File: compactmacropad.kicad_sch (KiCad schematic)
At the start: 31 parts, among them SW1 RotaryEncoder_Switch, SW3 RotaryEncoder_Switch, U1 MCU_Seeed_XIAO_RP2040, U2 SN74LV1T34DBV

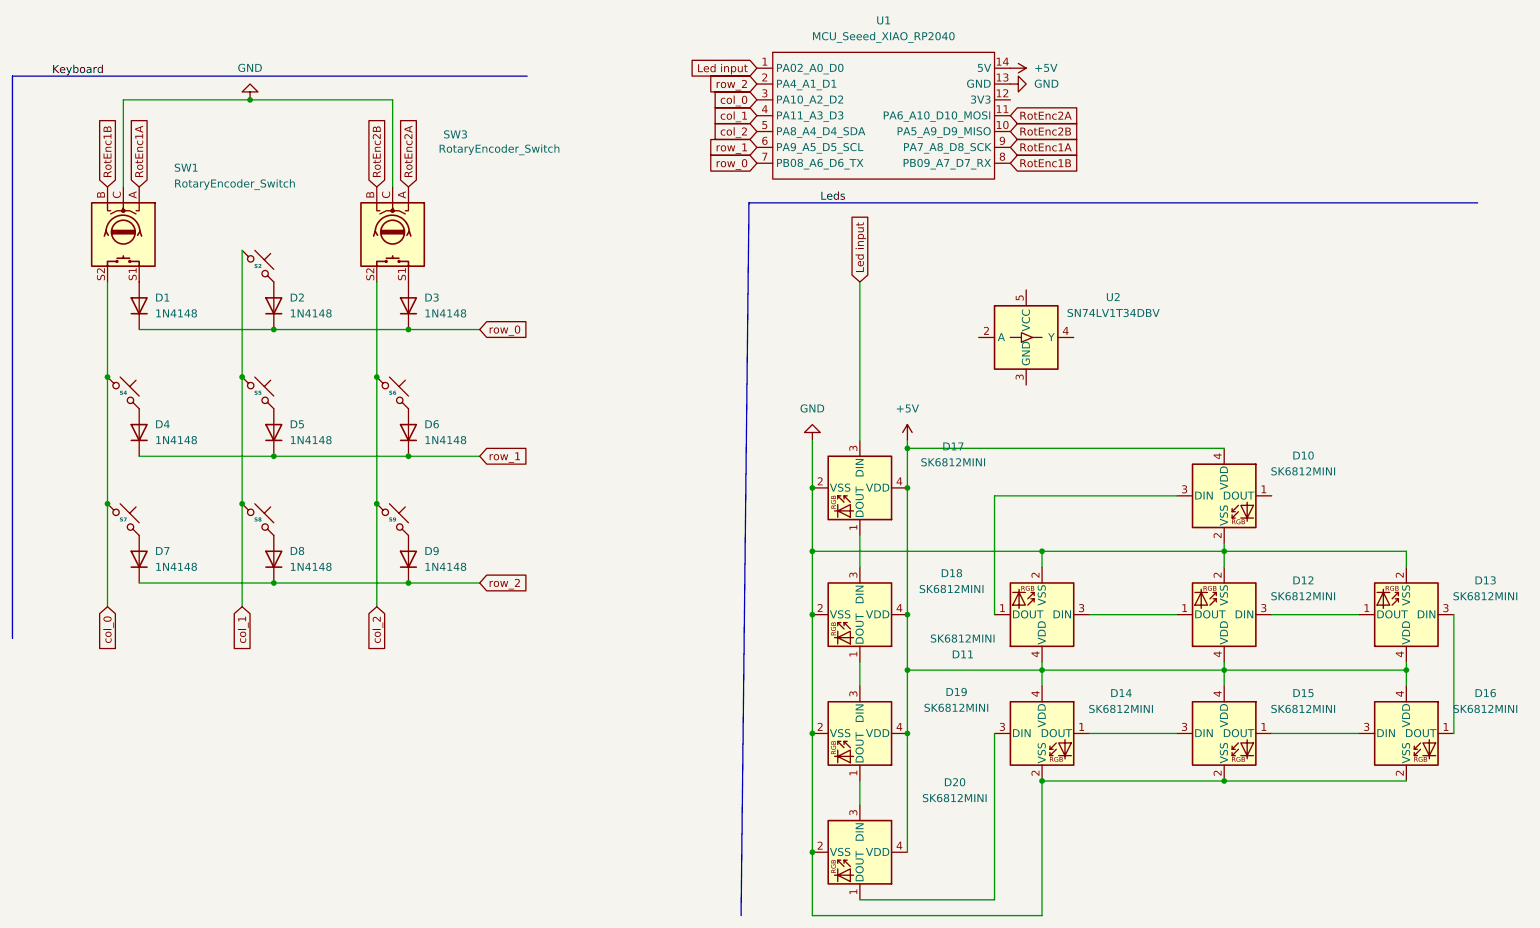
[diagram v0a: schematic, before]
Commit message: New files
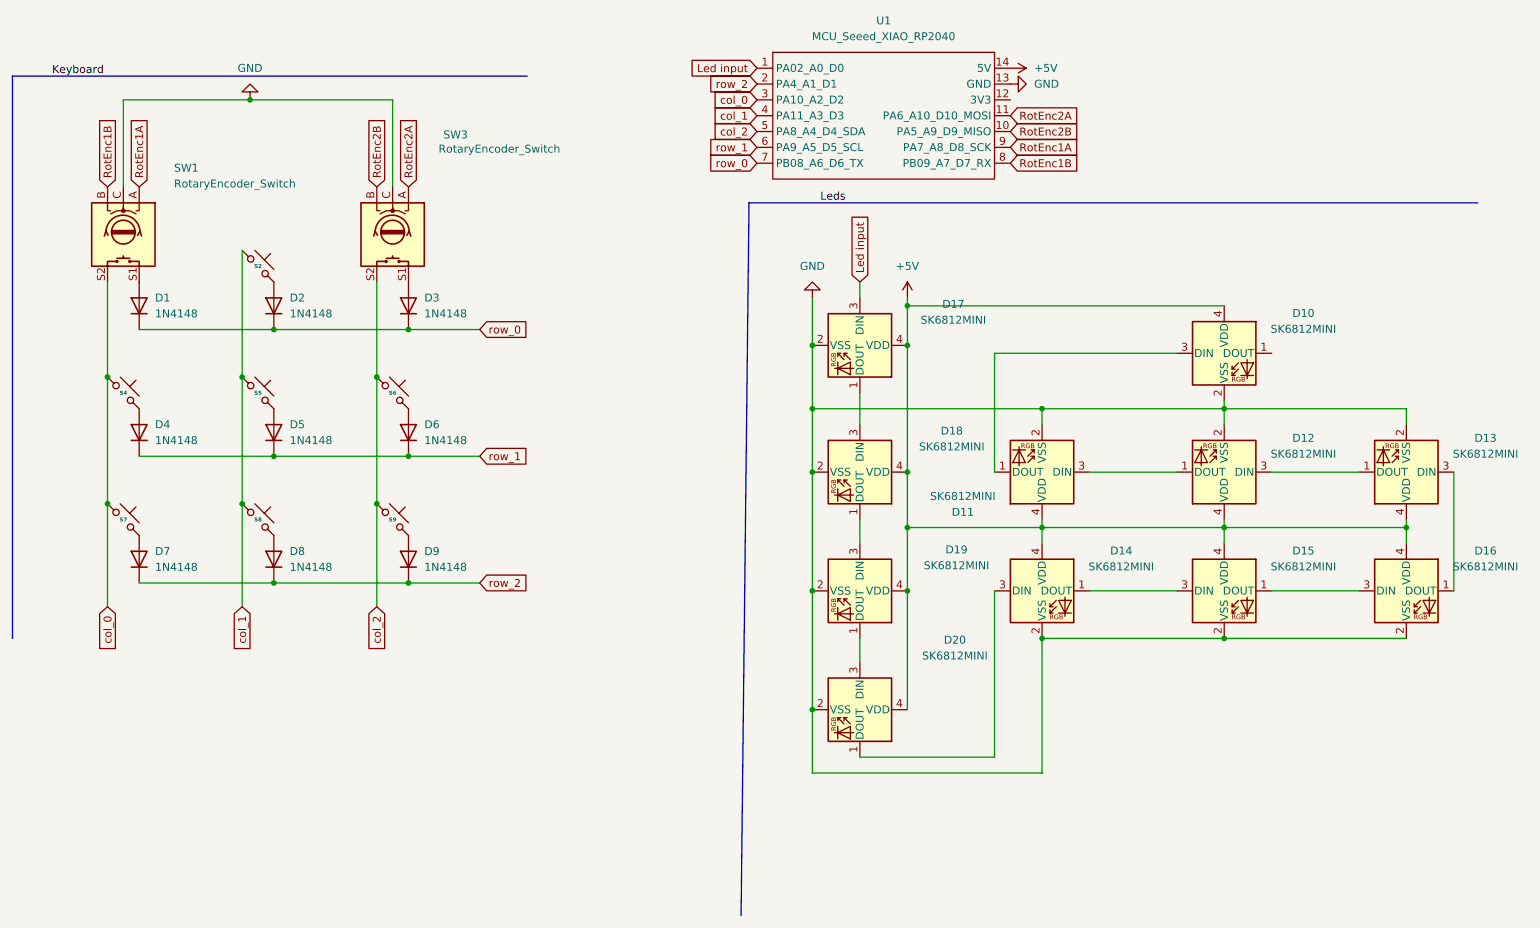
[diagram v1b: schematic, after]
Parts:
- removed U2: SN74LV1T34DBV, Package_TO_SOT_SMD:SOT-23-5, symbol Logic_LevelTranslator:SN74LV1T34DBV
- D10, D14, D15, D16: footprint LED_SMD:LED_SK6812MINI_PLCC4_3.5x3.5mm_P1.75mm -> kicad-keyboard-parts.pretty-master:MX_SK6812MINI-E_REV
- D11, D12, D13: footprint LED_SMD:LED_SK6812MINI_PLCC4_3.5x3.5mm_P1.75mm -> kicad-keyboard-parts.pretty-master:MX_SK6812MINI-E_REV_Rot
- D17, D18, D19, D20: footprint LED_SMD:LED_SK6812MINI_PLCC4_3.5x3.5mm_P1.75mm -> kicad-keyboard-parts.pretty-master:MX_SK6812MINI-E
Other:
- moved on the sheet: D10, D11, D12, D13, D14, D15, D16, D17, D18, D19, D20
